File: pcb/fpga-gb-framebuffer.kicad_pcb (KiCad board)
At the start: 2 copper layers, 74.9 x 45.7 mm, 20 parts

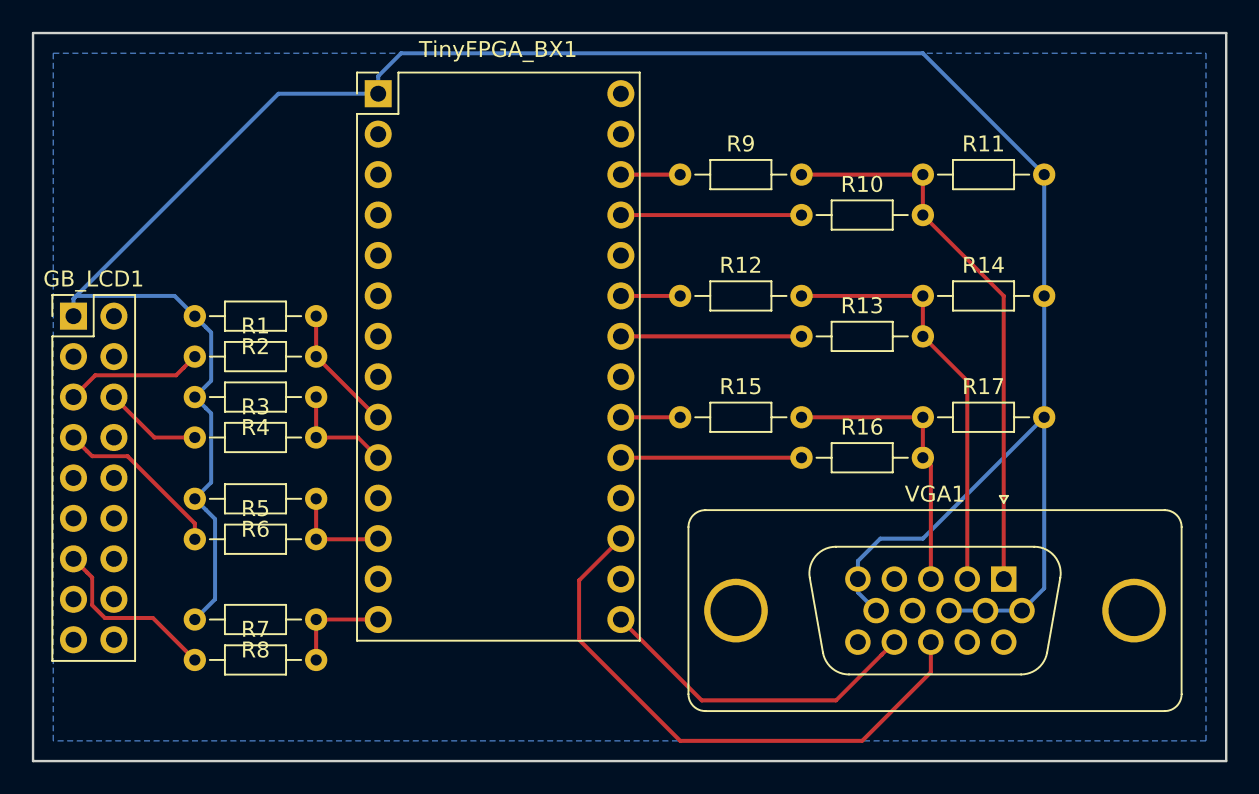
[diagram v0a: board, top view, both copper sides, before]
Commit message: Updated PCB design
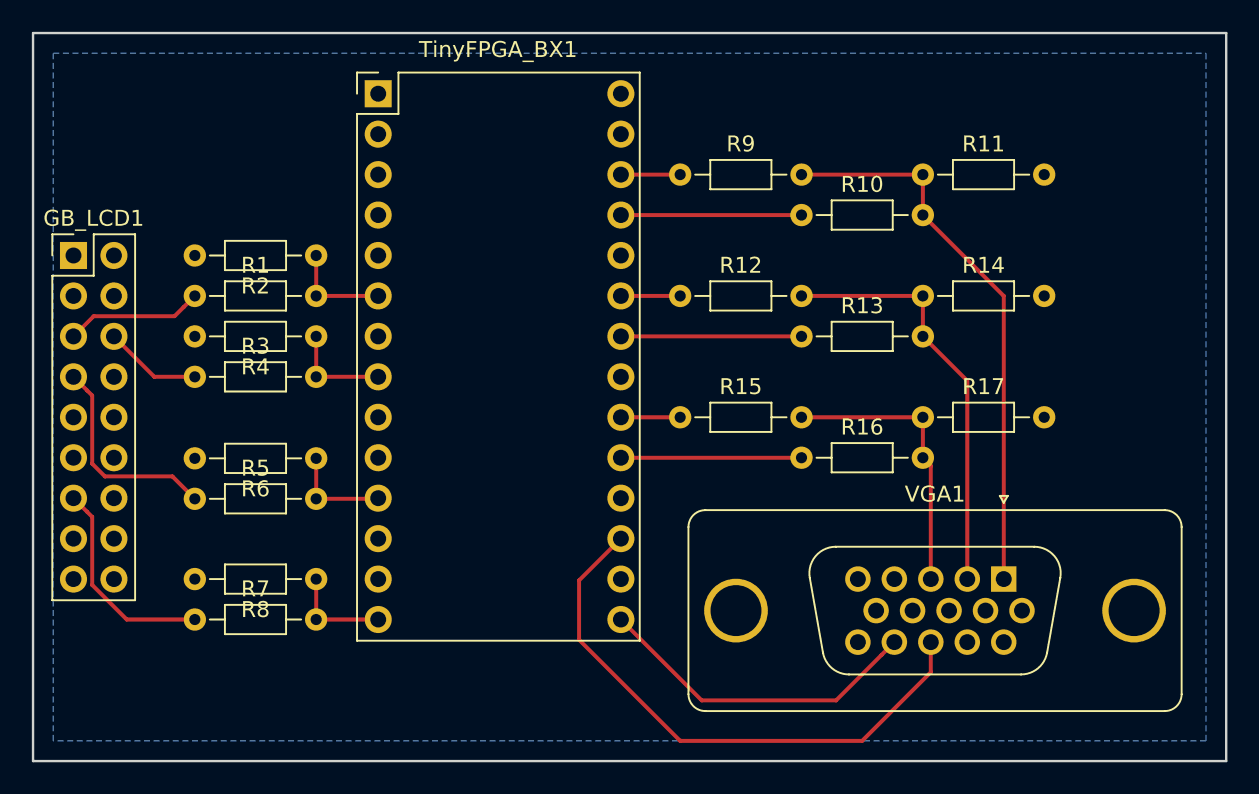
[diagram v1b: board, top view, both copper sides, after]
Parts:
- moved GB_LCD1 3.81 mm to (100.3, 69.8)
- moved R1 3.81 mm to (108.0, 72.4)
- moved R2 3.81 mm to (115.6, 69.8)
- moved R3 3.81 mm to (108.0, 77.5)
- moved R4 3.81 mm to (115.6, 74.9)
- moved R6 2.54 mm to (115.6, 82.6)
- moved R7 2.54 mm to (108.0, 92.7)
- moved R5 2.54 mm to (108.0, 85.1)
- moved R8 2.54 mm to (115.6, 90.2)
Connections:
- TinyFPGA_BX1 pad 10: IN_DATA_1 -> Net-(TinyFPGA_BX1-Pad10)
- TinyFPGA_BX1 pad 11: Net-(TinyFPGA_BX1-Pad11) -> IN_PIXEL_CLK
- TinyFPGA_BX1 pad 12: IN_PIXEL_CLK -> Net-(TinyFPGA_BX1-Pad12)
- TinyFPGA_BX1 pad 6: Net-(TinyFPGA_BX1-Pad6) -> IN_DATA_0
- TinyFPGA_BX1 pad 8: Net-(TinyFPGA_BX1-Pad8) -> IN_DATA_1
- TinyFPGA_BX1 pad 9: IN_DATA_0 -> Net-(TinyFPGA_BX1-Pad9)
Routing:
- net GB_GND: track 153.8 -> 0.00 mm
- net GB_PIXEL_CLK: track 10.8 -> 13.3 mm
- net GB_VSYNC: track 11.3 -> 13.3 mm
- net IN_DATA_0: track 8.01 -> 6.44 mm
- net IN_DATA_1: track 6.96 -> 6.44 mm
